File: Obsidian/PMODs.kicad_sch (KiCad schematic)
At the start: 6 parts, among them J14 Conn_02x06_Top_Bottom, J15 Conn_02x06_Top_Bottom, J4 Conn_02x06_Top_Bottom, J5 Conn_02x06_Top_Bottom, J6 Conn_02x06_Top_Bottom, J7 Conn_02x06_Top_Bottom

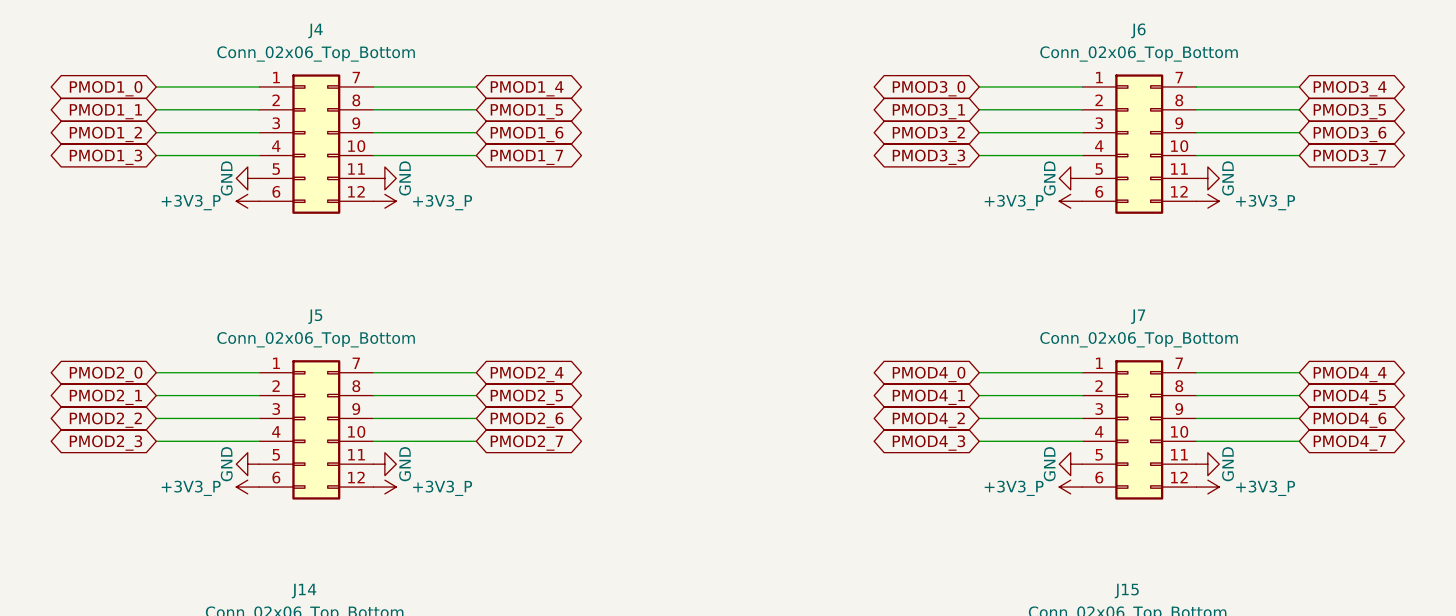
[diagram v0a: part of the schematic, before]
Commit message: revison v1.1.0 ready to review
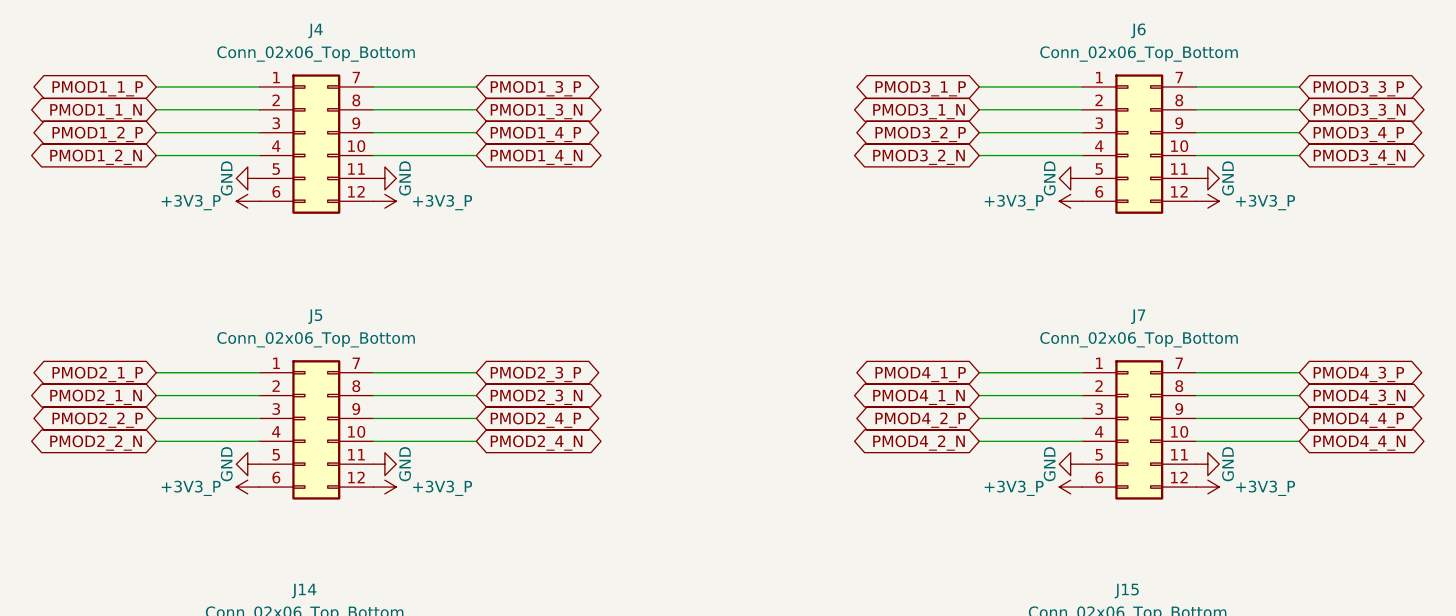
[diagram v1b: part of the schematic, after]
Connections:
- net PMOD1_0 renamed PMOD1_1_P
- net PMOD1_1 renamed PMOD1_1_N
- net PMOD1_2 renamed PMOD1_2_P
- net PMOD1_3 renamed PMOD1_2_N
- net PMOD1_4 renamed PMOD1_3_P
- net PMOD1_5 renamed PMOD1_3_N
- net PMOD1_6 renamed PMOD1_4_P
- net PMOD1_7 renamed PMOD1_4_N
- net PMOD2_0 renamed PMOD2_1_P
- net PMOD2_1 renamed PMOD2_1_N
- net PMOD2_2 renamed PMOD2_2_P
- net PMOD2_3 renamed PMOD2_2_N
- net PMOD2_4 renamed PMOD2_3_P
- net PMOD2_5 renamed PMOD2_3_N
- net PMOD2_6 renamed PMOD2_4_P
- net PMOD2_7 renamed PMOD2_4_N
- net PMOD3_0 renamed PMOD3_1_P
- net PMOD3_1 renamed PMOD3_1_N
- net PMOD3_2 renamed PMOD3_2_P
- net PMOD3_3 renamed PMOD3_2_N
- net PMOD3_4 renamed PMOD3_3_P
- net PMOD3_5 renamed PMOD3_3_N
- net PMOD3_6 renamed PMOD3_4_P
- net PMOD3_7 renamed PMOD3_4_N
- net PMOD4_0 renamed PMOD4_1_P
- net PMOD4_1 renamed PMOD4_1_N
- net PMOD4_2 renamed PMOD4_2_P
- net PMOD4_3 renamed PMOD4_2_N
- net PMOD4_4 renamed PMOD4_3_P
- net PMOD4_5 renamed PMOD4_3_N
- net PMOD4_6 renamed PMOD4_4_P
- net PMOD4_7 renamed PMOD4_4_N

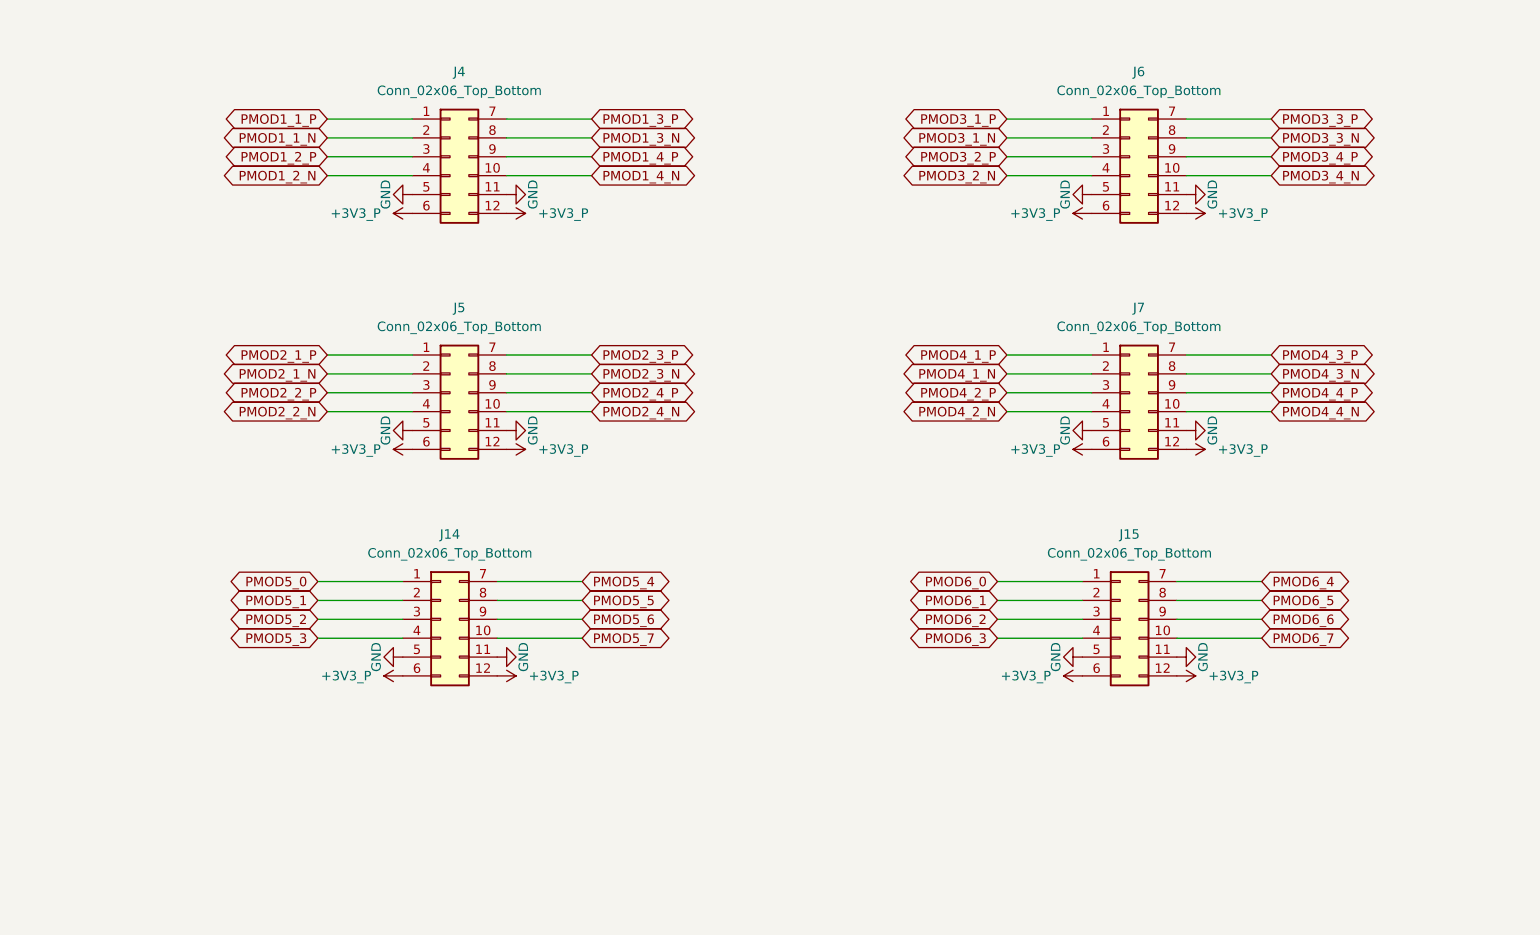
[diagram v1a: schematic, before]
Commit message: minor changes
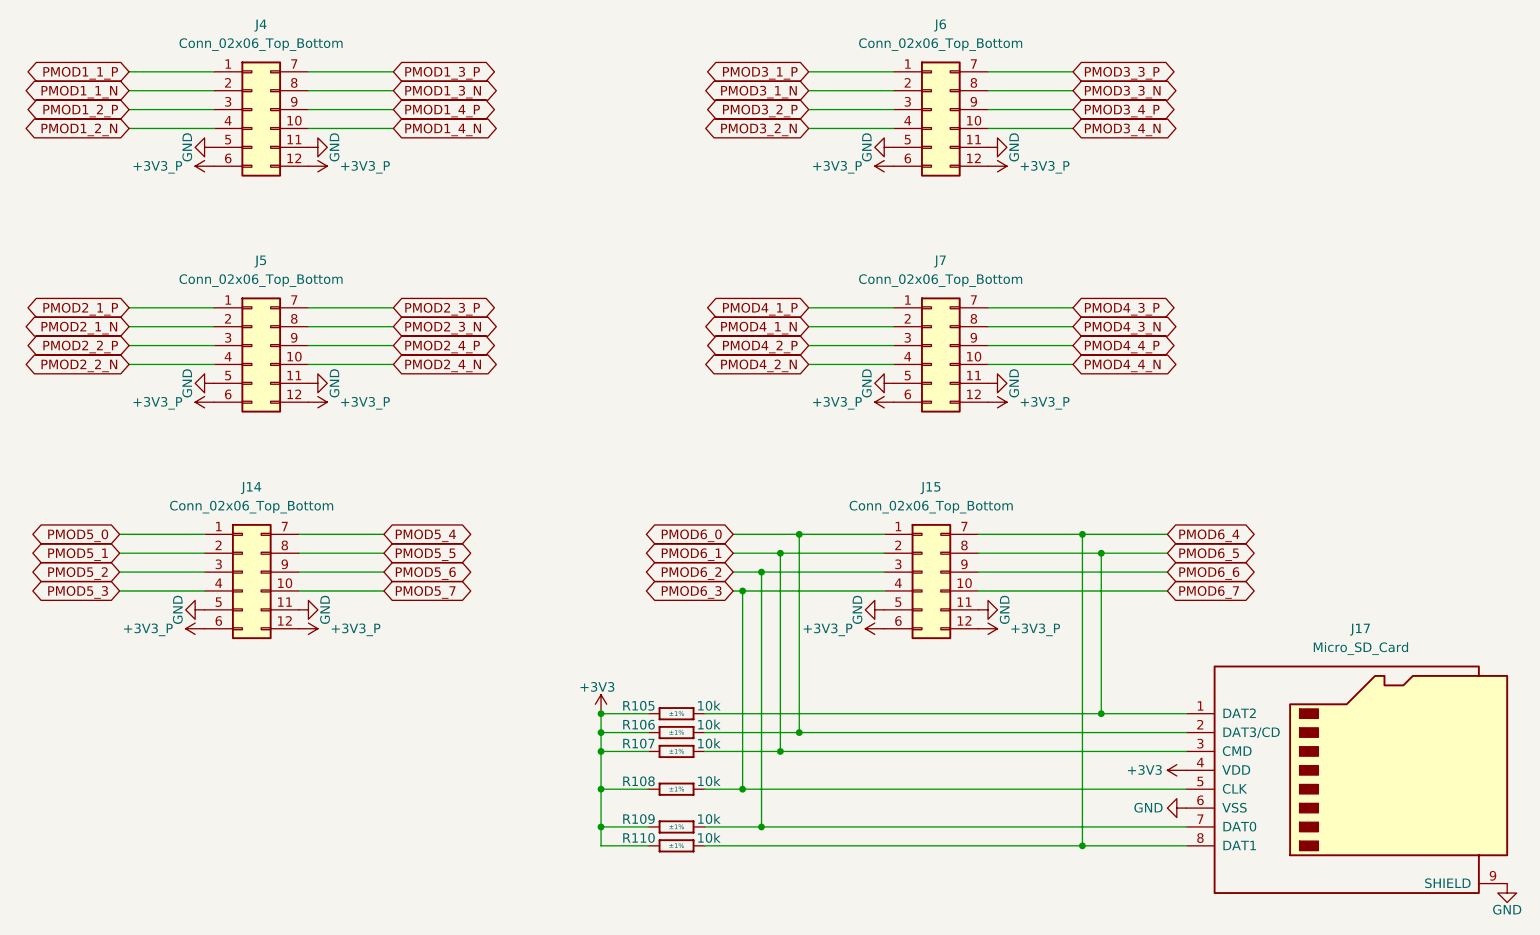
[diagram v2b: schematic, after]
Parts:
- added J17: Micro_SD_Card, Connector_Card:microSD_HC_Molex_47219-2001, symbol Connector:Micro_SD_Card
- added R105, R106, R107, R108, R109, R110: R0402_10K_1%_0.0625W_100PPM, Resistors SMD:RESC1005X40N, symbol Resistors SMD:R0402_10K_1%_0.0625W_100PPM
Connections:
- net GND: now also J17.6 (VSS), J17.9 (SHIELD)
- net PMOD6_0: now also J17.2 (DAT3/CD), R106.2
- net PMOD6_1: now also J17.3 (CMD), R107.2
- net PMOD6_2: now also J17.7 (DAT0), R109.2
- net PMOD6_3: now also J17.5 (CLK), R108.2
- net PMOD6_4: now also J17.8 (DAT1), R110.2
- net PMOD6_5: now also J17.1 (DAT2), R105.2
- new net +3V3: J17.4 (VDD), R105.1, R106.1, R107.1, R108.1, R109.1, R110.1
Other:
- moved on the sheet: J14, J15, J4, J5, J6, J7
